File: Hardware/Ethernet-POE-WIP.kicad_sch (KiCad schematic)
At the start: 16 parts, among them J1 Conn_01x07_Male, J2 Conn_01x04_Male, J3 Conn_01x02_Male, J4 Conn_01x02_Male, J5 Conn_01x02_Male, J6 Conn_01x02_Male, J7 Conn_01x08_Male, J9 QWIIC_Stackable

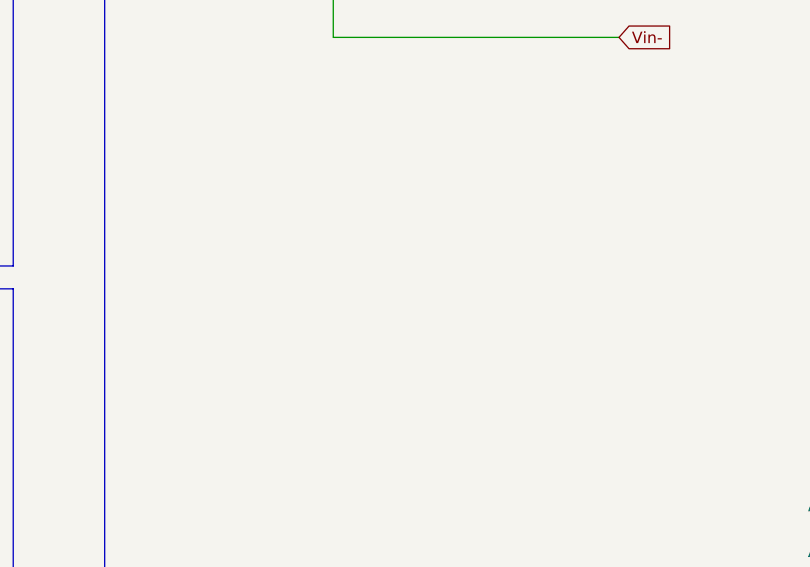
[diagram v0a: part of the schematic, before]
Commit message: More on POE...
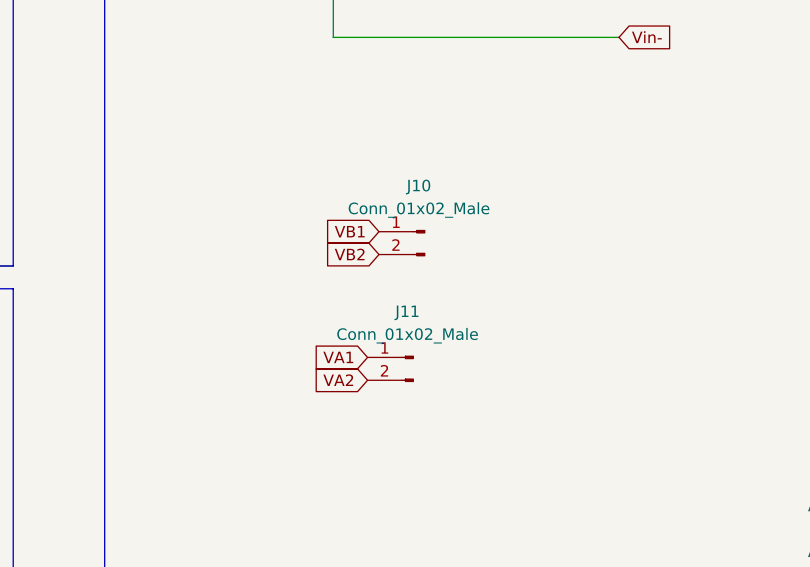
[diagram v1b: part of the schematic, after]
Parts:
- added J10, J11: Conn_01x02_Male, Tinker:Board_Stacker_2, symbol Connector:Conn_01x02_Male
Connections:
- net VA1: now also J11.1 (Pin_1)
- net VA2: now also J11.2 (Pin_2)
- net VB1: now also J10.1 (Pin_1)
- net VB2: now also J10.2 (Pin_2)
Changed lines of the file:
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@@
+    )
+  )
+  (global_label "VB2" (shape input) (at 146.05 105.41 180) (fields_autoplaced)
+    (effects (font (size 1.27 1.27)) (justify right))
+    (property "Intersheet References" "${INTERSHEET_REFS}" (id 0) (at 140.0688 105.3306 0)
+      (effects (font (size 1.27 1.27)) (justify right) hide)
     )
   )
@@
     (effects (font (size 1.27 1.27)) (justify right))
     (property "Intersheet References" "${INTERSHEET_REFS}" (id 0) (at 142.7902 59.6106 0)
+      (effects (font (size 1.27 1.27)) (justify right) hide)
+    )
+  )
+  (global_label "VA2" (shape input) (at 144.78 119.38 180) (fields_autoplaced)
+    (effects (font (size 1.27 1.27)) (justify right))
+    (property "Intersheet References" "${INTERSHEET_REFS}" (id 0) (at 138.9802 119.3006 0)
       (effects (font (size 1.27 1.27)) (justify right) hide)
     )
@@
     )
   )
+  (global_label "VB1" (shape input) (at 146.05 102.87 180) (fields_autoplaced)
+    (effects (font (size 1.27 1.27)) (justify right))
+    (property "Intersheet References" "${INTERSHEET_REFS}" (id 0) (at 140.0688 102.7906 0)
+      (effects (font (size 1.27 1.27)) (justify right) hide)
+    )
+  )
   (global_label "Vsec" (shape input) (at 53.34 172.72 180) (fields_autoplaced)
     (effects (font (size 1.27 1.27)) (justify right))
@@
     (effects (font (size 1.27 1.27)) (justify right))
     (property "Intersheet References" "${INTERSHEET_REFS}" (id 0) (at 168.7345 143.4306 0)
+      (effects (font (size 1.27 1.27)) (justify right) hide)
+    )
+  )
+  (global_label "VA1" (shape input) (at 144.78 116.84 180) (fields_autoplaced)
+    (effects (font (size 1.27 1.27)) (justify right))
+    (property "Intersheet References" "${INTERSHEET_REFS}" (id 0) (at 138.9802 116.7606 0)
       (effects (font (size 1.27 1.27)) (justify right) hide)
     )
@@
     (pin "1")
   )
+  (symbol (lib_id "Connector:Conn_01x02_Male") (at 149.86 116.84 0) (mirror y) (unit 1)
+    (in_bom no) (on_board yes)
+    (property "Reference" "J11" (id 0) (at 149.225 111.76 0))
+    (property "Value" "Conn_01x02_Male" (id 1) (at 149.225 114.3 0))
+    (property "Footprint" "Tinker:Board_Stacker_2" (id 2) (at 149.86 116.84 0)
+      (effects (font (size 1.27 1.27)) hide)
+    )
+    (property "Datasheet" "~" (id 3) (at 149.86 116.84 0)
+      (effects (font (size 1.27 1.27)) hide)
+    )
+    (pin "1")
+    (pin "2")
+  )
+  (symbol (lib_id "Connector:Conn_01x02_Male") (at 151.13 102.87 0) (mirror y) (unit 1)
+    (in_bom no) (on_board yes)
+    (property "Reference" "J10" (id 0) (at 150.495 97.79 0))
+    (property "Value" "Conn_01x02_Male" (id 1) (at 150.495 100.33 0))
+    (property "Footprint" "Tinker:Board_Stacker_2" (id 2) (at 151.13 102.87 0)
+      (effects (font (size 1.27 1.27)) hide)
+    )
+    (property "Datasheet" "~" (id 3) (at 151.13 102.87 0)
+      (effects (font (size 1.27 1.27)) hide)
+    )
+    (pin "1")
+    (pin "2")
+  )
   (symbol (lib_id "Diode_Bridge:MB4S") (at 153.67 46.99 0) (unit 1)
     (in_bom yes) (on_board yes) (fields_autoplaced)
@@
       (reference "J9") (unit 1) (value "QWIIC_Stackable") (footprint "Tinker:QWIIC_Stack_II")
     )
+    (path "/8af4d545-763d-455d-b107-3627fdce1d98"
+      (reference "J10") (unit 1) (value "Conn_01x02_Male") (footprint "Tinker:Board_Stacker_2")
+    )
+    (path "/8991d857-4568-4b0a-a10b-61c40f80b916"
+      (reference "J11") (unit 1) (value "Conn_01x02_Male") (footprint "Tinker:Board_Stacker_2")
+    )
     (path "/012e9a98-7cf1-409d-a24d-6f21f0c7188f"
